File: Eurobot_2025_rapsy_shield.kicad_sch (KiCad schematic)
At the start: 30 parts, among them J1 Raspberry_Pi_2_3, J2 SPI, J4 Conn_01x02, J5 AU, J6 Conn_01x04, Q1 2N7002, Q2 2N7002, U1 TPS54302

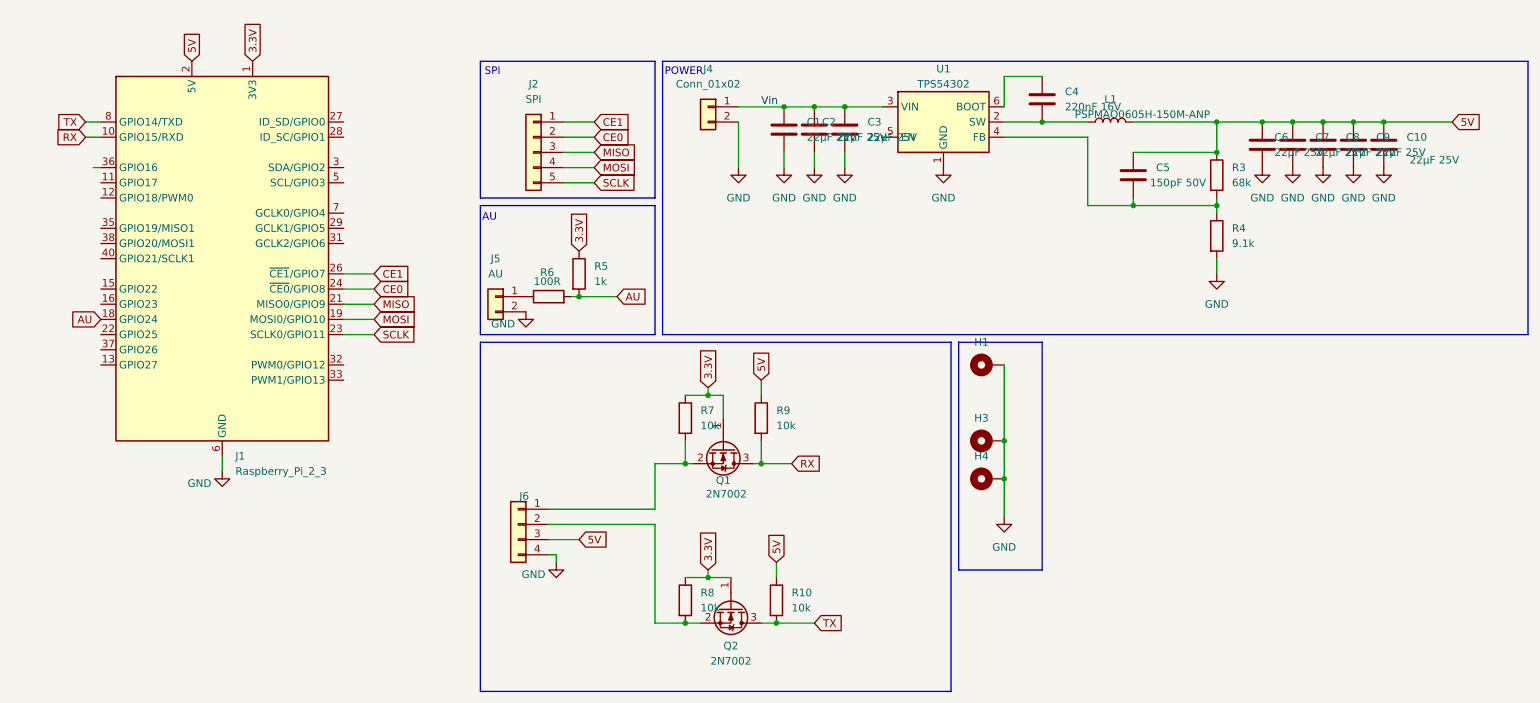
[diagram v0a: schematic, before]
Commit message: v1 ok
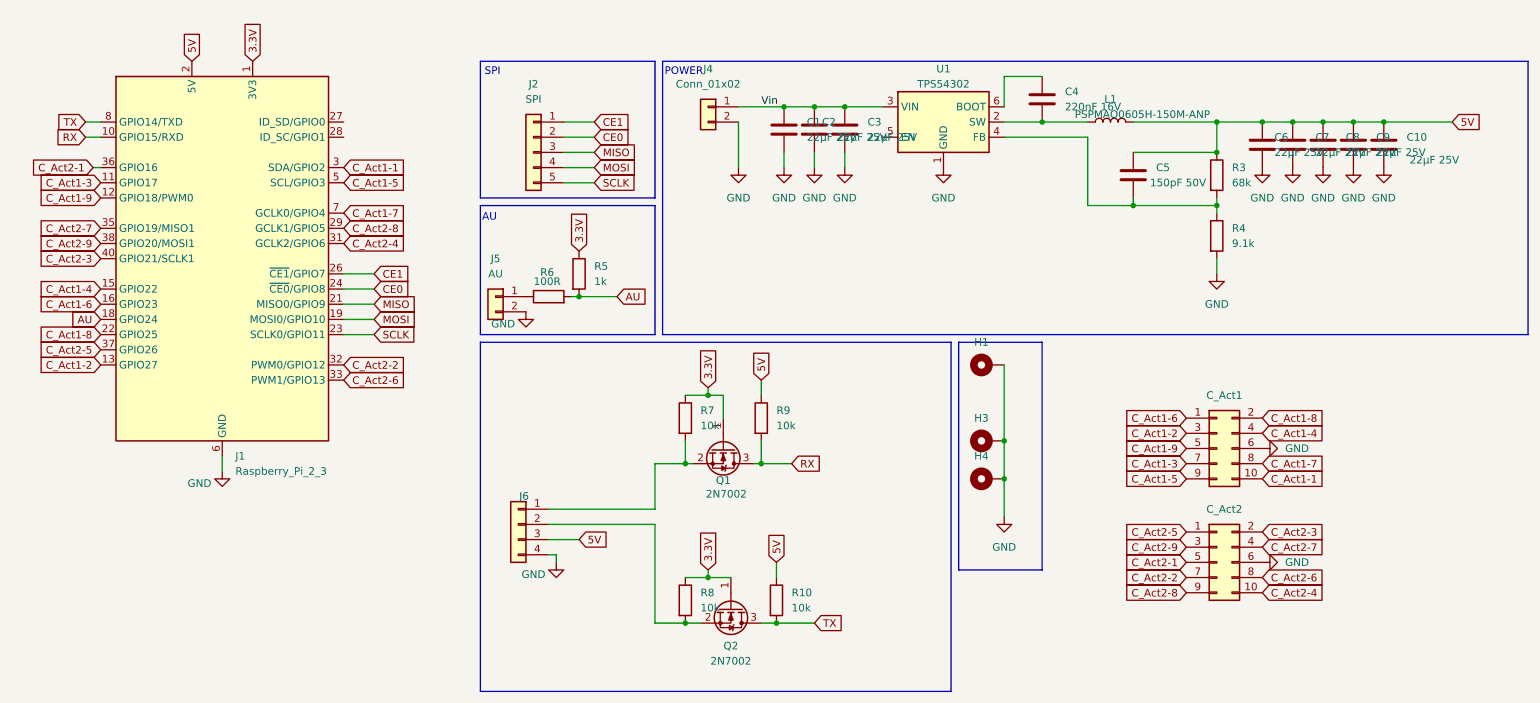
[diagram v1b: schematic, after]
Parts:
- added C_Act1, C_Act2: Conn_02x05_Odd_Even, Connector_IDC:IDC-Header_2x05_P2.54mm_Vertical, symbol Connector_Generic:Conn_02x05_Odd_Even
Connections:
- net GND: now also C_Act1.6 (Pin_6), C_Act2.6 (Pin_6)
- net C_Act1-3: now reaches J1.11 (GPIO17)
- net C_Act1-3: now also C_Act1.7 (Pin_7)
- net C_Act1-9: now reaches J1.12 (GPIO18/PWM0)
- net C_Act1-9: now also C_Act1.5 (Pin_5)
- net C_Act1-2: now reaches J1.13 (GPIO27)
- net C_Act1-2: now also C_Act1.3 (Pin_3)
- net C_Act1-4: now reaches J1.15 (GPIO22)
- net C_Act1-4: now also C_Act1.4 (Pin_4)
- net C_Act1-6: now reaches J1.16 (GPIO23)
- net C_Act1-6: now also C_Act1.1 (Pin_1)
- net C_Act1-8: now reaches J1.22 (GPIO25)
- net C_Act1-8: now also C_Act1.2 (Pin_2)
- net C_Act2-8: now reaches J1.29 (GCLK1/GPIO5)
- net C_Act2-8: now also C_Act2.9 (Pin_9)
- net C_Act1-1: now reaches J1.3 (SDA/GPIO2)
- net C_Act1-1: now also C_Act1.10 (Pin_10)
- net C_Act2-4: now reaches J1.31 (GCLK2/GPIO6)
- net C_Act2-4: now also C_Act2.10 (Pin_10)
- net C_Act2-2: now reaches J1.32 (PWM0/GPIO12)
- net C_Act2-2: now also C_Act2.7 (Pin_7)
- net C_Act2-6: now reaches J1.33 (PWM1/GPIO13)
- net C_Act2-6: now also C_Act2.8 (Pin_8)
- net C_Act2-7: now reaches J1.35 (GPIO19/MISO1)
- net C_Act2-7: now also C_Act2.4 (Pin_4)
- net C_Act2-1: now reaches J1.36 (GPIO16)
- net C_Act2-1: now also C_Act2.5 (Pin_5)
- net C_Act2-5: now reaches J1.37 (GPIO26)
- net C_Act2-5: now also C_Act2.1 (Pin_1)
- net C_Act2-9: now reaches J1.38 (GPIO20/MOSI1)
- net C_Act2-9: now also C_Act2.3 (Pin_3)
- net C_Act2-3: now reaches J1.40 (GPIO21/SCLK1)
- net C_Act2-3: now also C_Act2.2 (Pin_2)
- net C_Act1-5: now reaches J1.5 (SCL/GPIO3)
- net C_Act1-5: now also C_Act1.9 (Pin_9)
- net C_Act1-7: now reaches J1.7 (GCLK0/GPIO4)
- net C_Act1-7: now also C_Act1.8 (Pin_8)
